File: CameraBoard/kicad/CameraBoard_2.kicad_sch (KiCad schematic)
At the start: 40 parts, among them Q2 BVSS123LT1G, Q3 BSS84, U4 TS5A3159ADBVR, U5 ICM7242IBAZ-SMD, U6 H11F1SR2M, U7 H11F1SR2M, U8 SN74LVC1G17DCKR

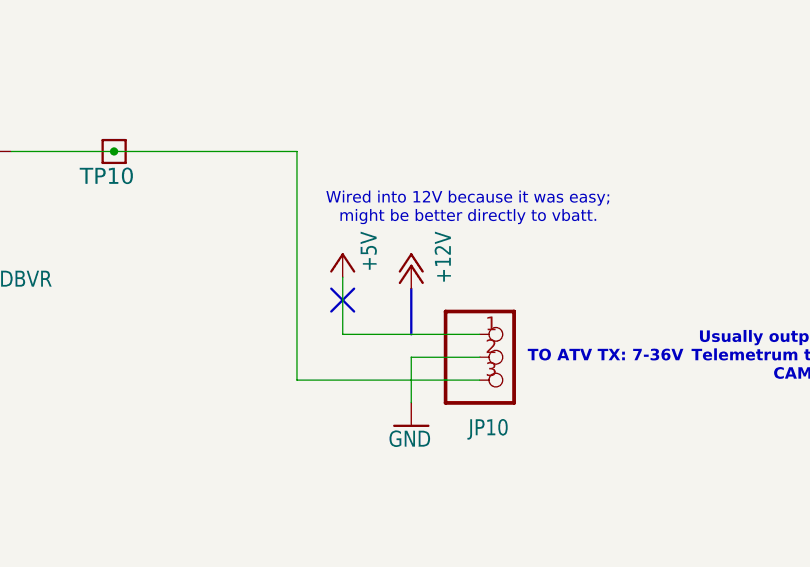
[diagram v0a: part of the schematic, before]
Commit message: Minor updates to PCB
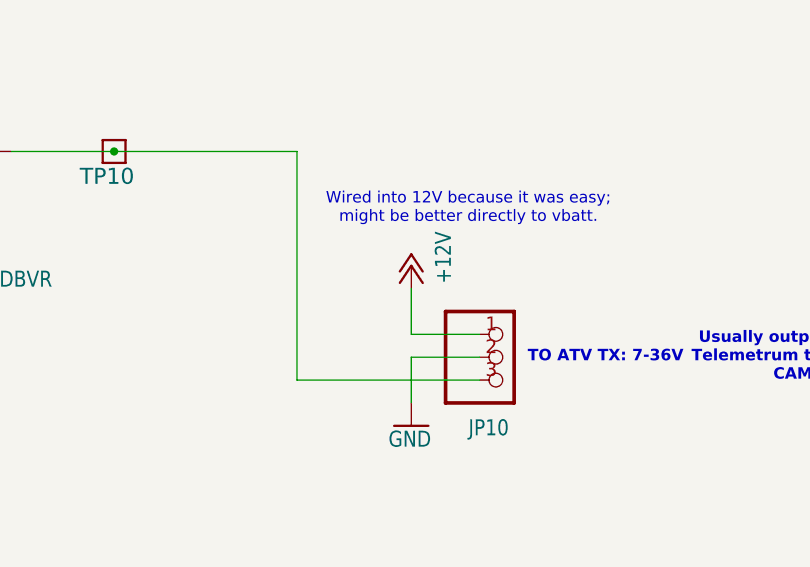
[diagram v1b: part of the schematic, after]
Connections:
- net +12V: now also JP10.1
- net +5V: no longer JP10.1
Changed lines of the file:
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@@
 	(wire
 		(pts
-			(xy 196.85 231.14) (xy 212.09 231.14)
-		)
-		(stroke
-			(width 0.1524)
-			(type solid)
-		)
-	)
-	(wire
-		(pts
 			(xy 191.77 236.22) (xy 212.09 236.22)
 		)
@@
 	(wire
 		(pts
+			(xy 204.47 226.06) (xy 204.47 231.14)
+		)
+		(stroke
+			(width 0)
+			(type default)
+		)
+	)
+	(wire
+		(pts
 			(xy 88.9 200.66) (xy 88.9 207.01)
 		)
@@
 	(wire
 		(pts
-			(xy 196.85 224.79) (xy 196.85 231.14)
-		)
-		(stroke
-			(width 0.1524)
-			(type solid)
-		)
-	)
-	(wire
-		(pts
 			(xy 299.72 182.88) (xy 299.72 181.61)
 		)
@@
 	(wire
 		(pts
+			(xy 212.09 231.14) (xy 204.47 231.14)
+		)
+		(stroke
+			(width 0)
+			(type default)
+		)
+	)
+	(wire
+		(pts
 			(xy 88.9 207.01) (xy 88.9 213.36)
 		)
@@
 	(polyline
 		(pts
-			(xy 195.58 226.06) (xy 198.12 228.6)
-		)
-		(stroke
-			(width 0.254)
-			(type solid)
-			(color 255 0 0 1)
-		)
-	)
-	(polyline
-		(pts
 			(xy 116.84 88.9) (xy 129.54 88.9)
 		)
@@
 		)
 	)
-	(polyline
-		(pts
-			(xy 195.58 228.6) (xy 198.12 226.06)
-		)
-		(stroke
-			(width 0.254)
-			(type solid)
-			(color 255 0 0 1)
-		)
-	)
 	(wire
 		(pts
@@
 		)
 	)
-	(polyline
-		(pts
-			(xy 204.47 231.14) (xy 204.47 226.06)
-		)
-		(stroke
-			(width 0.254)
-			(type solid)
-			(color 255 0 0 1)
-		)
-	)
 	(wire
 		(pts
@@
 					(unit 1)
 				)
-			)
-		)
-	)
-	(symbol
-		(lib_id "CameraBoard-eagle-import:+5V")
-		(at 196.85 222.25 0)
-		(unit 1)
-		(exclude_from_sim no)
-		(in_bom yes)
-		(on_board yes)
-		(dnp no)
-		(property "Reference" "#P+2"
-			(at 196.85 222.25 0)
-			(effects
-				(font
-					(size 1.27 1.27)
-				)
-				(hide yes)
-			)
-		)
-		(property "Value" "+5V"
-			(at 198.755 219.71 90)
-			(effects
-				(font
-					(size 1.778 1.5113)
-				)
-				(justify right top)
-			)
-		)
-		(property "Footprint" ""
-			(at 196.85 222.25 0)
-			(effects
-				(font
-					(size 1.27 1.27)
-				)
-				(hide yes)
-			)
-		)
-		(property "Datasheet" ""
-			(at 196.85 222.25 0)
-			(effects
-				(font
-					(size 1.27 1.27)
-				)
-				(hide yes)
-			)
-		)
-		(property "Description" ""
-			(at 196.85 222.25 0)
-			(effects
-				(font
-					(size 1.27 1.27)
-				)
-				(hide yes)
-			)
-		)
-		(pin "1"
-		)
-		(instances
-			(project "CameraBoard"
-				(path "/876601fa-fbd1-4e2d-9c28-84441865735b/537433a0-7b0a-4286-9b5c-a2c4a7e302ab"
-					(reference "#P+2")
-					(unit 1)
-				)
